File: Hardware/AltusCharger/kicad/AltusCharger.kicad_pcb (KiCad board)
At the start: 2 copper layers, 76.2 x 50.8 mm, 71 parts, among them J1 Conn_01x02_Socket, J2 Conn_01x02_Socket, J3 USB_C_Receptacle_USB2.0_16P, J4 Conn_01x02_Socket, J5 Conn_01x02_Socket, J6 Conn_01x02_Socket, J7 Conn_01x02_Socket, Q1 AO3401A, Q2 AO3400A, Q3 AO3400A, SW1 SSSS811101, U1 MCP73831-2-OT, U2 MCP73831-2-OT, U3 MCP73831-2-OT, U4 MCP73831-2-OT, U5 MCP73831-2-OT, U6 MCP73831-2-OT

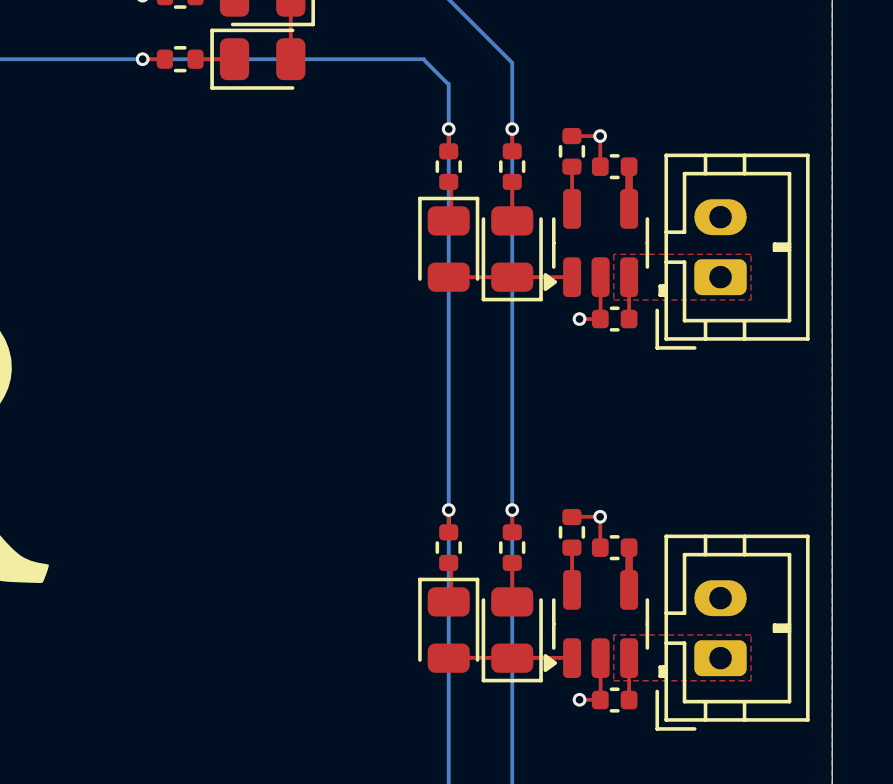
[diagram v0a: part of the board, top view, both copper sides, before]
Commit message: Altus Charger changes to gen fab files
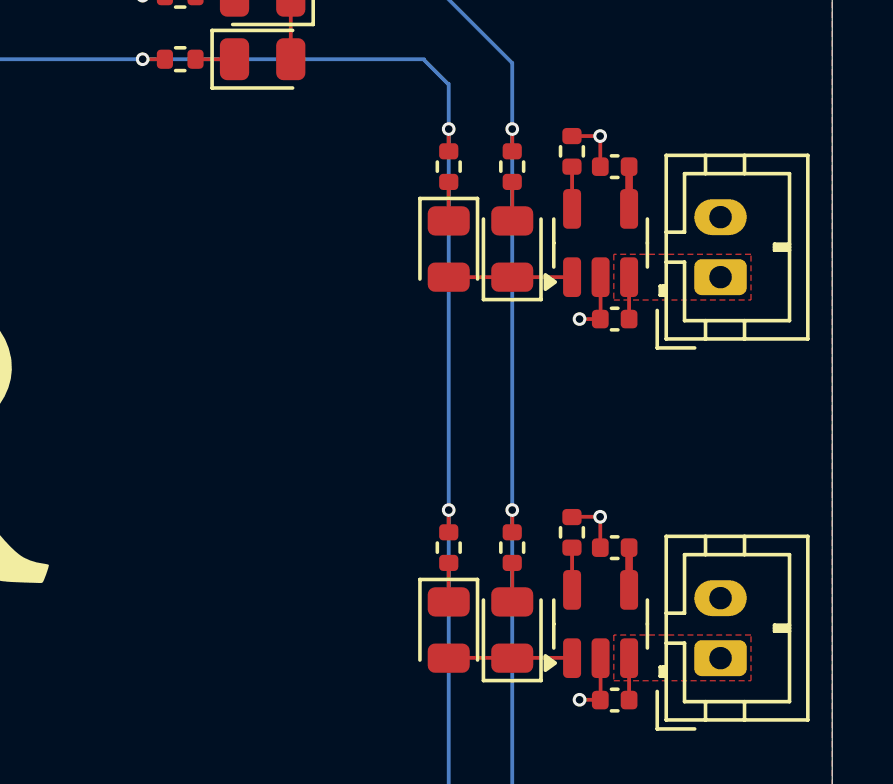
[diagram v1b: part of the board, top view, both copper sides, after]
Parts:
- removed D14, D15: KT-0805G, LED_SMD:LED_0805_2012Metric
- added D6: KT-0805R, LED_SMD:LED_0805_2012Metric, F.Cu at (167.1, 108.0)
- added D7: KT-0805R, LED_SMD:LED_0805_2012Metric, F.Cu at (167.1, 95.3)
- D10, D11: value KT-0805G -> KT-0805R
- D12, D13, D8, D9: value KT-0805R -> KT-0805G
- R10, R11, R18, R19, R4, R5: value 1k -> 510
- moved D11 45.1 mm to (120.7, 86.9), turned to 180 degrees
- moved D10 22.0 mm to (158.8, 86.9), turned to 180 degrees
- moved D8 2.12 mm to (165.0, 108.0), turned to -90 degrees
- moved D9 2.12 mm to (165.0, 95.3), turned to -90 degrees
- moved D12 2.12 mm to (158.8, 89.0), turned to 0 degrees
- moved D13 2.12 mm to (120.7, 89.0), turned to 0 degrees
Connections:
- D12 pad 2: Net-(D12-A) -> Net-(D10-K)
- D13 pad 2: Net-(D13-A) -> Net-(D11-K)
- D8 pad 1: Net-(D10-A) -> Net-(D8-K)
- D8 pad 2: Net-(D8-A) -> Net-(D6-K)
- D9 pad 1: Net-(D11-A) -> Net-(D9-K)
- D9 pad 2: Net-(D9-A) -> Net-(D7-K)
- R10 pad 1: Net-(D8-A) -> Net-(D6-A)
- R11 pad 1: Net-(D9-A) -> Net-(D7-A)
- R15 pad 1: Net-(D10-K) -> Net-(D8-K)
- R16 pad 1: Net-(D11-K) -> Net-(D9-K)
- R18 pad 1: Net-(D12-A) -> Net-(D10-A)
- R19 pad 1: Net-(D13-A) -> Net-(D11-A)
- R22 pad 1: Net-(D14-K) -> Net-(D12-K)
- R23 pad 1: Net-(D15-K) -> Net-(D13-K)
- U3 pad 1: Net-(D10-A) -> Net-(D6-K)
- U4 pad 1: Net-(D11-A) -> Net-(D7-K)
- U5 pad 1: Net-(D12-K) -> Net-(D10-K)
- U6 pad 1: Net-(D13-K) -> Net-(D11-K)
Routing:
- net Net-(D7-K): track 0.00 -> 3.94 mm
- net Net-(D6-K): track 0.00 -> 3.94 mm
- net Net-(D11-A): track 3.94 -> 1.30 mm
- net Net-(D13-K): track 3.94 -> 1.30 mm
- net Net-(D11-K): track 1.30 -> 3.94 mm
- net Net-(D10-K): track 1.30 -> 3.94 mm
- net Net-(D10-A): track 3.94 -> 1.30 mm
- net Net-(D12-K): track 3.94 -> 1.30 mm
- net Net-(D8-K): track 0.00 -> 1.37 mm
- net Net-(D14-K): track 1.30 -> 0.00 mm
- net Net-(D12-A): track 1.30 -> 0.00 mm
- net Net-(D9-K): track 0.00 -> 1.30 mm
- net Net-(D9-A): track 1.30 -> 0.00 mm
- net Net-(D8-A): track 1.30 -> 0.00 mm
- net Net-(D7-A): track 0.00 -> 1.30 mm
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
